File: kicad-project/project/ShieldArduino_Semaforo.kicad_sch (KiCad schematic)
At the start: 97 parts, among them IC1 TLIN1039DDFRQ1, IC2 TPS563200DDCR, IC3 MCP4901T-E_MS, J2 Conn_01x18, K1 RELAY, P1 Power, P2 Analog, P3 Digital, P4 Digital, P5 CONN_01X01, P6 CONN_01X01, P7 CONN_01X01, P8 CONN_01X01, Q1 PMOS, Q2 NMOS, Q3 NMOS, Q4 NMOS, Q5 NMOS, U1 MCP2542FD-E/MF, U3 LM4040DBZ-2.0

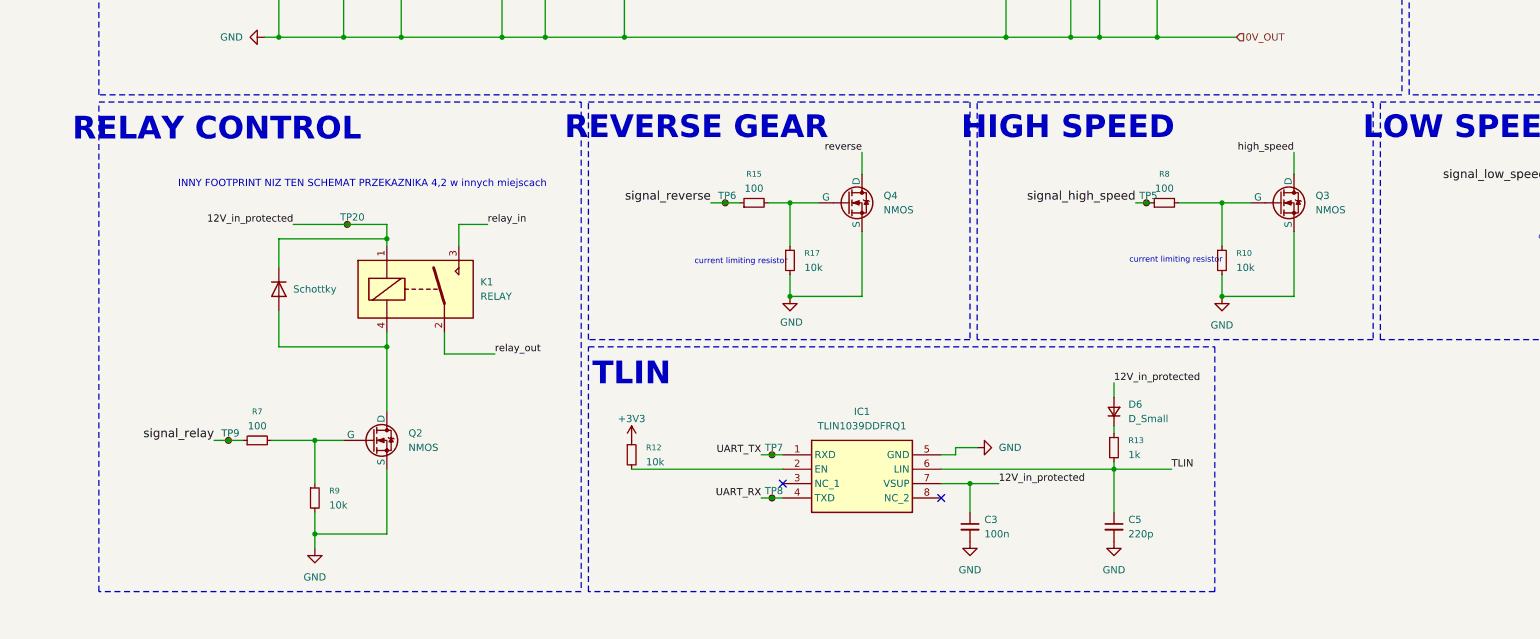
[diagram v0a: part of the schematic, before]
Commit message: kciad-schematic-tlin
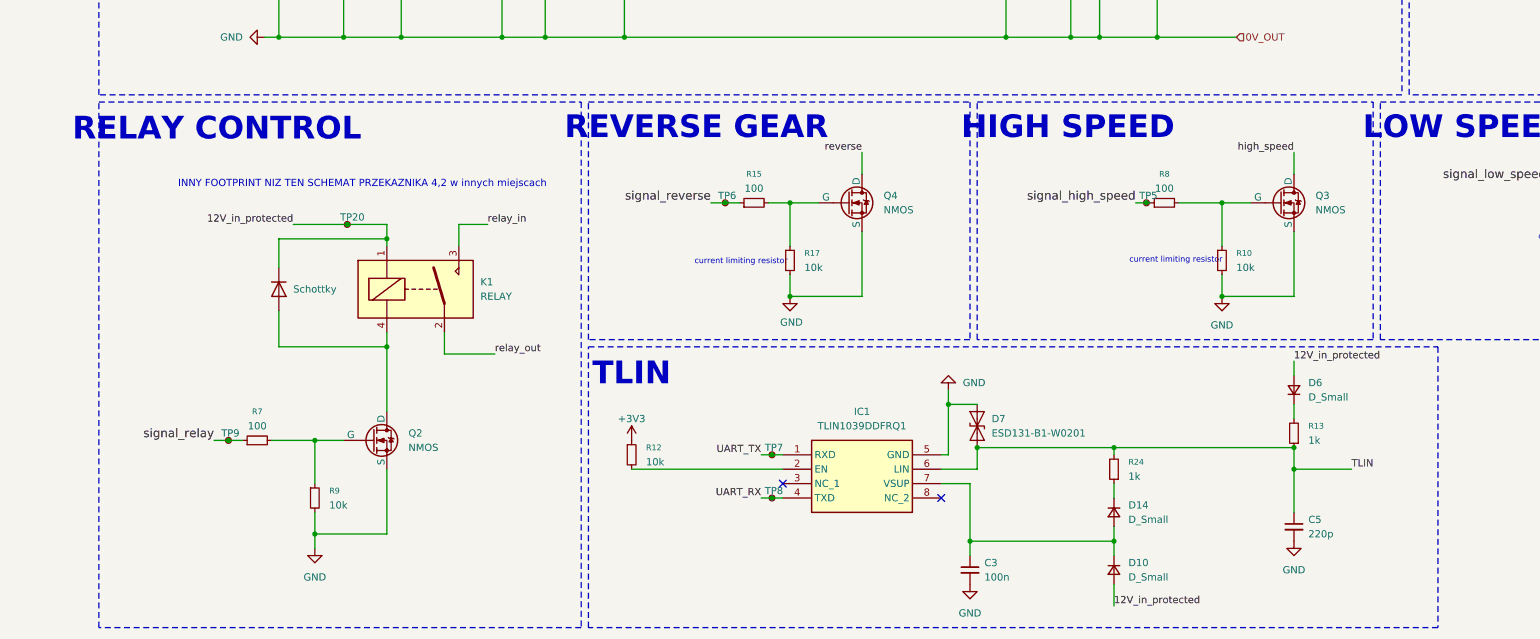
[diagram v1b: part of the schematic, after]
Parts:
- added D10, D14: D_Small, symbol Device:D_Small
- added D7: ESD131-B1-W0201, Diode_SMD:Infineon_SG-WLL-2-3_0.58x0.28_P0.36mm, symbol Diode:ESD131-B1-W0201
- added R24: 1k, Resistor_SMD:R_0805_2012Metric_Pad1.20x1.40mm_HandSolder, symbol Device:R_Small
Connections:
- net 12V_in_protected: now also D10.2 (A); no longer C3.1, IC1.7 (VSUP)
- net GND: now also D7.2 (A2)
- net TLIN: now also R13.1, D7.1 (A1), R24.2; no longer R13.2
- net at D6.1 (K): now also R13.2; no longer R13.1
- new net: C3.1, D10.1 (K), D14.2 (A), IC1.7 (VSUP)
- new net: D14.1 (K), R24.1
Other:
- moved on the sheet: C3, C5, D6
